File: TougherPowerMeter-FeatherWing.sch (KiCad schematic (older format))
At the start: 40 parts, among them J1 Jumper, J10 796639-2, J11 Jumper, J2 796639-2, J3 796639-2, J4 796639-2, J5 796639-2, J6 796639-2, J7 796639-2, J8 796639-2, J9 796639-2, U1 AP63205, U2 TPS1HB08A-Q1, U3 FeatherWing, U4 INA3221

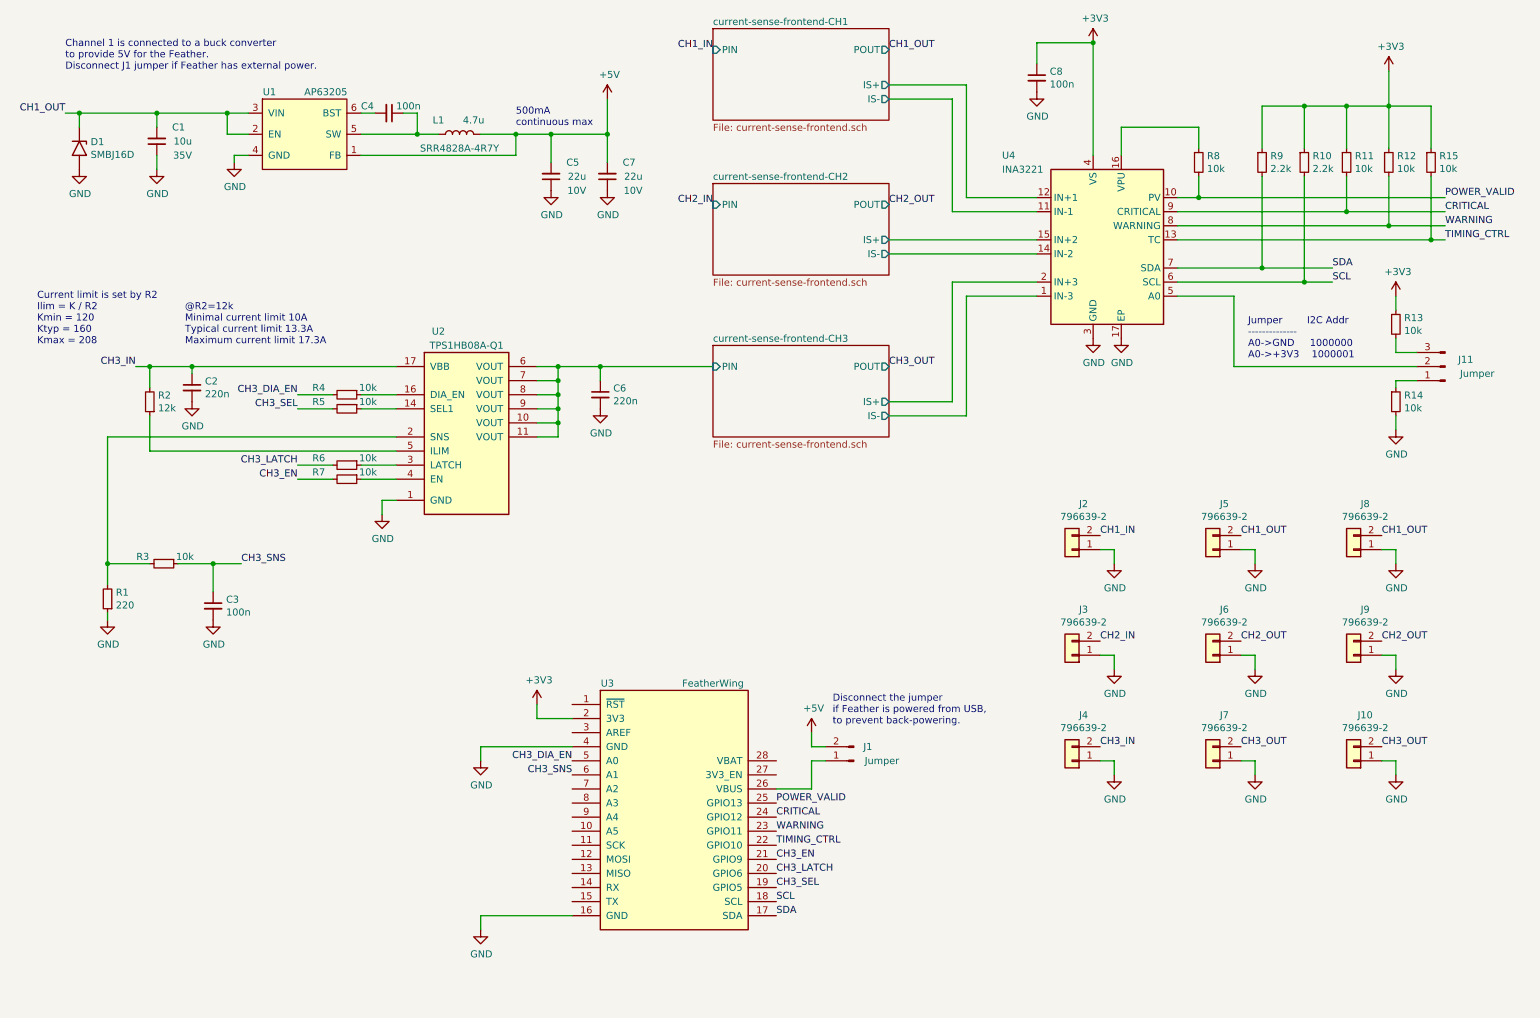
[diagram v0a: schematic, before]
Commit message: Finish design
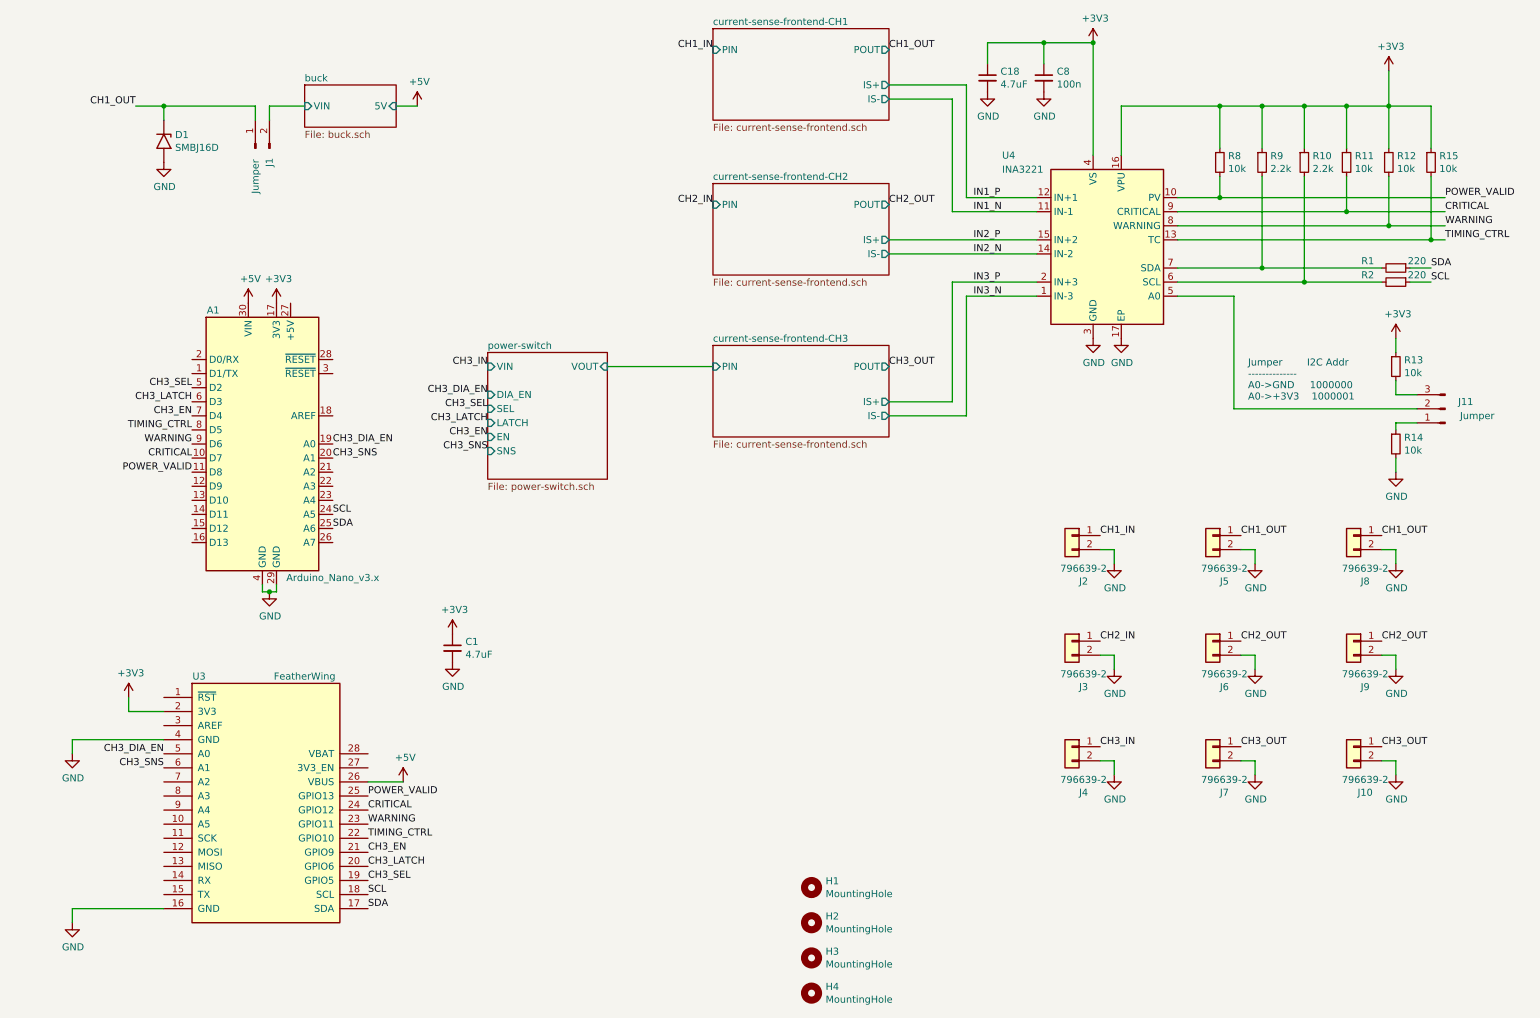
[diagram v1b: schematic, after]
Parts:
- removed C2, C6: 220n, Capacitor_SMD:C_0603_1608Metric, symbol Device:C_Small
- removed C3, C4: 100n, Resistor_SMD:R_0603_1608Metric, symbol Device:C_Small
- removed C5, C7: 22u, Capacitor_SMD:C_0805_2012Metric, symbol Device:C_Small
- removed L1: 4.7u, Inductor_SMD_BD:L_Bourns_SRR1210A, symbol Device:L
- removed R3, R4, R5, R6, R7: 10k, Resistor_SMD:R_0603_1608Metric, symbol Device:R_Small
- removed U1: AP63205, Package_TO_SOT_SMD:TSOT-23-6, symbol Power_Management_BD:AP63205
- removed U2: TPS1HB08A-Q1, Package_SO:HTSSOP-16-1EP_4.4x5mm_P0.65mm_EP3.4x5mm, symbol Power_Management_BD:TPS1HB08-Q1
- added A1: Arduino_Nano_v3.x, Module_BD:Arduino_Nano_NoSilk, symbol MCU_Module:Arduino_Nano_v3.x
- added C18: 4.7uF, Capacitor_SMD:C_0603_1608Metric, symbol Device:C_Small
- added H1, H2, H3, H4: MountingHole, MountingHole:MountingHole_3.2mm_M3_Pad_Via, symbol Mechanical:MountingHole
- C1: value 10u -> 4.7uF; footprint Capacitor_SMD:C_1206_3216Metric -> Capacitor_SMD:C_0603_1608Metric; Voltage 35V -> (none)
- R2: value 12k -> 220
- U3: footprint Module_BD:FeatherWing -> Module_BD:FeatherWing_NoMH
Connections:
- net +3V3: now also C1.1, R8.1, U4.16 (VPU), A1.17 (3V3), C18.1
- net +5V: now also U3.26 (VBUS), A1.30 (VIN); no longer J1.2 (Pin_2)
- net CH1_IN: now also J2.1 (Pin_1); no longer J2.2 (Pin_2)
- net CH1_OUT: now also J1.1 (Pin_1), J5.1 (Pin_1), J8.1 (Pin_1); no longer C1.2, J5.2 (Pin_2), J8.2 (Pin_2)
- net CH2_IN: now also J3.1 (Pin_1); no longer J3.2 (Pin_2)
- net CH2_OUT: now also J6.1 (Pin_1), J9.1 (Pin_1); no longer J6.2 (Pin_2), J9.2 (Pin_2)
- net CH3_DIA_EN: now also A1.19 (A0)
- net CH3_EN: now also A1.7 (D4)
- net CH3_IN: now also J4.1 (Pin_1); no longer J4.2 (Pin_2), R2.2
- net CH3_LATCH: now also A1.6 (D3)
- net CH3_OUT: now also J10.1 (Pin_1), J7.1 (Pin_1); no longer J10.2 (Pin_2), J7.2 (Pin_2)
- net CH3_SEL: now also A1.5 (D2)
- net CH3_SNS: now also A1.20 (A1)
- net CRITICAL: now also A1.10 (D7)
- net GND: now also C1.2, J10.2 (Pin_2), J2.2 (Pin_2), J3.2 (Pin_2), J4.2 (Pin_2), J5.2 (Pin_2), J6.2 (Pin_2), J7.2 (Pin_2), J8.2 (Pin_2), J9.2 (Pin_2), A1.29 (GND), A1.4 (GND), C18.2; no longer C1.1, J10.1 (Pin_1), J2.1 (Pin_1), J3.1 (Pin_1), J4.1 (Pin_1), J5.1 (Pin_1), J6.1 (Pin_1), J7.1 (Pin_1), J8.1 (Pin_1), J9.1 (Pin_1), R1.1
- net POWER_VALID: now also A1.11 (D8)
- net SCL: now also R2.1, A1.24 (A5); no longer R10.2, U4.6 (SCL)
- net SDA: now also R1.1, A1.25 (A6); no longer R9.2, U4.7 (SDA)
- net TIMING_CTRL: now also A1.8 (D5)
- net WARNING: now also A1.9 (D6)
- net at R1.2: now also R9.2, U4.7 (SDA)
- net current-sense-frontend-CH1/IS+ renamed IN1_P
- net current-sense-frontend-CH1/IS- renamed IN1_N
- net current-sense-frontend-CH2/IS+ renamed IN2_P
- net current-sense-frontend-CH2/IS- renamed IN2_N
- net current-sense-frontend-CH3/IS+ renamed IN3_P
- net current-sense-frontend-CH3/IS- renamed IN3_N
- new net: R10.2, R2.2, U4.6 (SCL)
- new net buck/VIN: J1.2 (Pin_2)
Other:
- note removed: "500mA \ncontinuous max"
- note removed: "@R2=12k\nMinimal current limit 10A\nTypical current limit 13.3A\nMaximum current limit 17.3A"
- note removed: "Channel 1 is connected to a buck converter \nto provide 5V for the Feather.\nDisconnect J1 jumper if Feather has external power."
- note removed: "Current limit is set by R2\nIlim = K / R2\nKmin = 120\nKtyp = 160\nKmax = 208"
- note removed: "Disconnect the jumper\nif Feather is powered from USB,\nto prevent back-powering."
- moved on the sheet: C8, J11, R13, R14, R8, U3
